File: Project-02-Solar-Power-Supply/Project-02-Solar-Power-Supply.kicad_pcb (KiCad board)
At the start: 2 copper layers, 39.1 x 20.3 mm, 17 parts, among them J1 Conn_01x02_Pin, J2 Conn_01x02_Pin, J3 Conn_01x02_Pin, J4 Conn_01x02_Pin, Q1 2N7002, U1 AP3015AKTR-G1

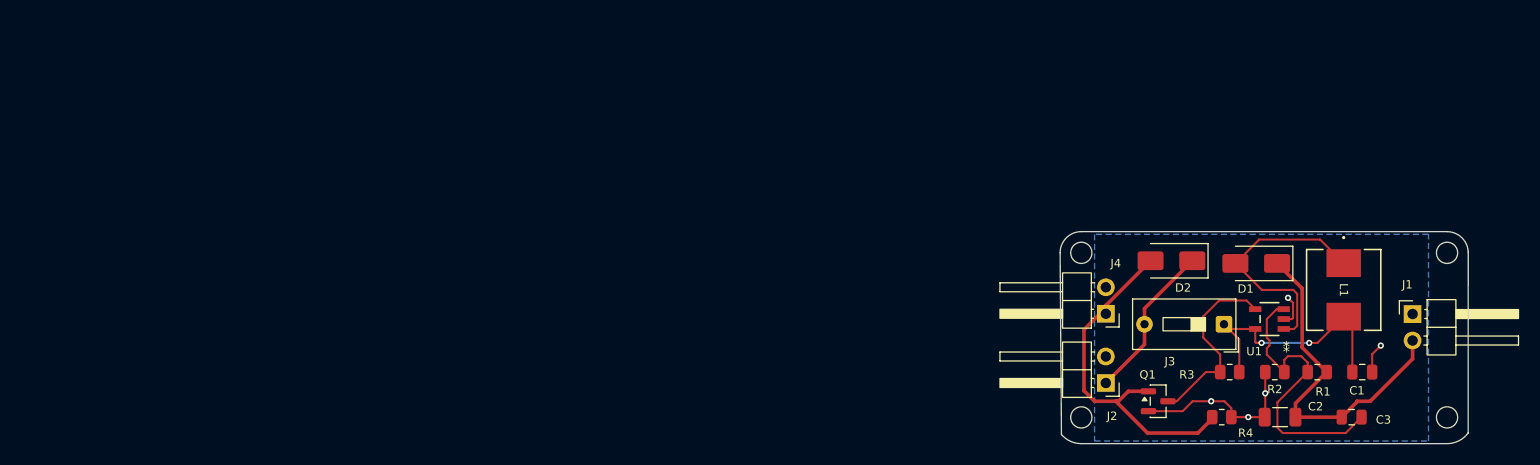
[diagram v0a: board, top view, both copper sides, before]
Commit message: small update
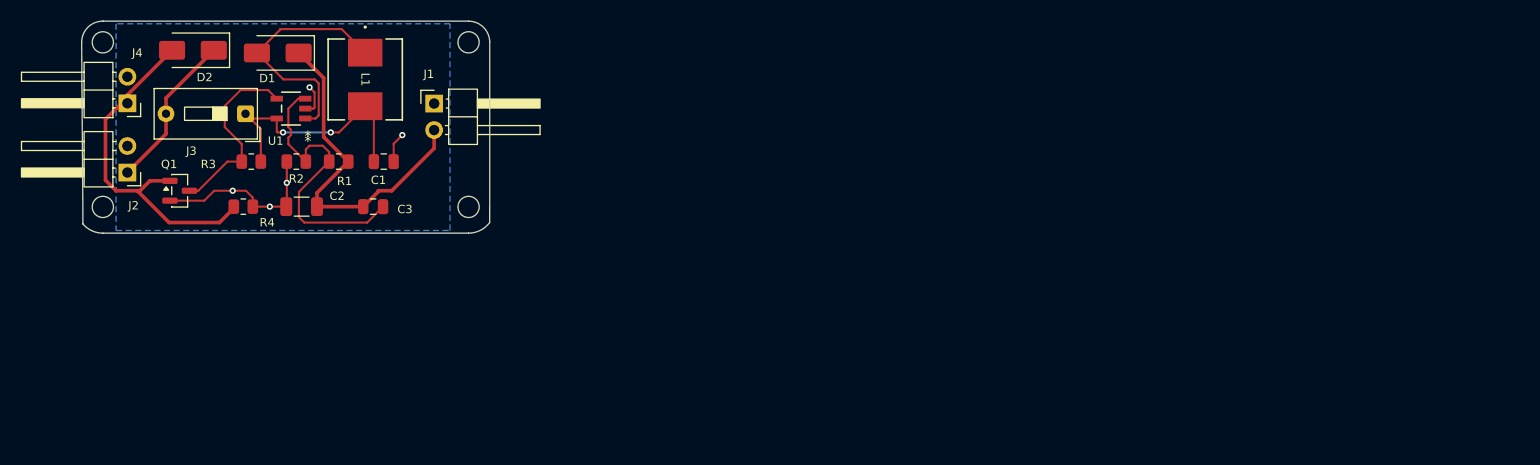
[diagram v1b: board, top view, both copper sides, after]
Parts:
- moved C1 95.9 mm to (88.6, 69.5)
- moved D2 95.9 mm to (70.3, 58.8)
- moved J1 95.9 mm to (93.4, 63.9)
- moved R1 95.9 mm to (84.3, 69.5)
- moved R2 95.9 mm to (80.2, 69.5)
- moved REF** 95.9 mm to (82.8, 68.4)
- moved C2 95.9 mm to (80.7, 73.8)
- moved C3 95.9 mm to (87.6, 73.8)
- moved D1 95.9 mm to (78.4, 59.1)
- moved J3 95.9 mm to (75.3, 64.9)
- moved J4 95.9 mm to (64.0, 63.9)
- moved L1 95.9 mm to (86.8, 61.6)
- moved Q1 95.9 mm to (69.0, 72.3)
- moved R3 95.9 mm to (75.9, 69.5)
- moved R4 95.9 mm to (75.1, 73.8)
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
